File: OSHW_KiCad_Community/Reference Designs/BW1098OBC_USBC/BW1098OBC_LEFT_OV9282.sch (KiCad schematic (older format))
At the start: 20 parts, among them J2 BBR43-24KB533 for camera modu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

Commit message: Hierarchical pin/label/text fixes, ground/power nets fixed
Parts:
- C10, C11, C12, C7, C8, C9: symbol BW1098OBC_TopLevel-rescue:BW1098OBC_IMX378-rescue_GRM188R61A106ME69D--BW1098OBC_IMX378-SchDoc-rescue-BW1098OBC_IMX378-c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 -> depthAI_sch:GRM188R61A106ME69D
- FB4, FB5, FB6: symbol BW1098OBC_TopLevel-rescue:BW1098OBC_IMX378-rescue_2508056017Y2--BW1098OBC_IMX378-SchDoc-rescue-BW1098OBC_IMX378-cache -> depthAI_sch:2508056017Y2
- J2: symbol BW1098OBC_TopLevel-rescue:BW1098OBC_LEFT_OV9282-SchDoc-rescue_TG161B-201_Connector--BW1098OBC_LEFT_OV9282-cache -> depthAI_sch:TG161B-201_Connector
- R10, R4, R5, R6, R7, R8, R9: symbol BW1098OBC_TopLevel-rescue:BW1098OBC_LEFT_OV9282-SchDoc-rescue_CRCW06030000Z0EA--BW1098OBC_LEFT_OV9282-cache -> depthAI_sch:CRCW06030000Z0EA
- R11, R3: symbol BW1098OBC_TopLevel-rescue:BW1098OBC_IMX378-rescue_RC0402FR-1310KL--BW1098OBC_IMX378-SchDoc-rescue-BW1098OBC_IMX378-cache -> depthAI_sch:RC0402FR-1310KL
- R12: symbol BW1098OBC_TopLevel-rescue:BW1098OBC_LEFT_OV9282-SchDoc-rescue_CRCW04020000Z0ED--BW1098OBC_LEFT_OV9282-cache -> depthAI_sch:CRCW04020000Z0ED
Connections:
- net labels removed: FSIN1_IN, Parameter Set, Power_trace
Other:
- note added: "Parameter Set\nPower Trace"
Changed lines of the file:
@@
 Comment4 ""
 $EndDescr
-Text Label 9800 5800 0    60   ~ 0
+Text Label 10400 5800 0    60   ~ 0
 STROBE1
 Text Notes 6600 900  0    60   ~ 0
@@
 Text Label 13500 3600 0    60   ~ 0
 I2C2_SCL
-Text Label 9800 5200 0    60   ~ 0
+Text Label 10300 5200 0    60   ~ 0
 I2C2_SDA
-Text Label 9800 5100 0    60   ~ 0
+Text Label 10300 5100 0    60   ~ 0
 I2C2_SCL
 Text Notes 800  6550 0    60   ~ 0
@@
 	1    0    0    -1
 $EndComp
-Text Label 9800 5400 0    60   ~ 0
-FSIN1_IN
-Text Label 7150 7050 1    70   ~ 0
-Parameter Set
-Text Label 7250 7050 1    70   ~ 0
-Power_trace
-Text Label 8450 7050 1    70   ~ 0
-Parameter Set
-Text Label 8550 7050 1    70   ~ 0
-Power_trace
-Text Label 9750 7050 1    70   ~ 0
-Parameter Set
-Text Label 9850 7050 1    70   ~ 0
-Power_trace
 Text Label 9440 7440 0    70   ~ 0
 10V
@@
 	10300 5200 9300 5200
 Wire Wire Line
-	9300 4800 10300 4800
-Wire Wire Line
 	7500 5200 6200 5200
 Wire Wire Line
@@
 Wire Wire Line
 	800  6650 1500 6650
-Wire Wire Line
-	11400 5400 11000 5400
 Wire Wire Line
 	13300 3600 14100 3600
@@
 Connection ~ 9650 7450
 $Comp
-L BW1098OBC_TopLevel-rescue:BW1098OBC_IMX378-rescue_2508056017Y2--BW1098OBC_IMX378-SchDoc-rescue-BW1098OBC_IMX378-cache FB4
+L depthAI_sch:2508056017Y2 FB4
 U 1 1 5FD53040
 P 1400 1000
@@
 $EndComp
 $Comp
-L BW1098OBC_TopLevel-rescue:BW1098OBC_IMX378-rescue_GRM188R61A106ME69D--BW1098OBC_IMX378-SchDoc-rescue-BW1098OBC_IMX378-cache C8
+L depthAI_sch:GRM188R61A106ME69D C8
 U 1 1 5FD5303F
 P 7450 7350
@@
 $EndComp
 $Comp
-L BW1098OBC_TopLevel-rescue:BW1098OBC_IMX378-rescue_GRM188R61A106ME69D--BW1098OBC_IMX378-SchDoc-rescue-BW1098OBC_IMX378-cache C7
+L depthAI_sch:GRM188R61A106ME69D C7
 U 1 1 5FD5303E
 P 6850 7350
@@
 $EndComp
 $Comp
-L BW1098OBC_TopLevel-rescue:BW1098OBC_IMX378-rescue_GRM188R61A106ME69D--BW1098OBC_IMX378-SchDoc-rescue-BW1098OBC_IMX378-cache C9
+L depthAI_sch:GRM188R61A106ME69D C9
 U 1 1 5FD5303D
 P 8150 7350
@@
 $EndComp
 $Comp
-L BW1098OBC_TopLevel-rescue:BW1098OBC_LEFT_OV9282-SchDoc-rescue_TG161B-201_Connector--BW1098OBC_LEFT_OV9282-cache J2
+L depthAI_sch:TG161B-201_Connector J2
 U 1 1 5FD5303C
 P 7500 4800
@@
 $EndComp
 $Comp
-L BW1098OBC_TopLevel-rescue:BW1098OBC_LEFT_OV9282-SchDoc-rescue_CRCW06030000Z0EA--BW1098OBC_LEFT_OV9282-cache R4
+L depthAI_sch:CRCW06030000Z0EA R4
 U 1 1 5FD5303B
 P 2000 6150
@@
 $EndComp
 $Comp
-L BW1098OBC_TopLevel-rescue:BW1098OBC_LEFT_OV9282-SchDoc-rescue_CRCW06030000Z0EA--BW1098OBC_LEFT_OV9282-cache R7
+L depthAI_sch:CRCW06030000Z0EA R7
 U 1 1 5FD5303A
 P 2500 6150
@@
 $EndComp
 $Comp
-L BW1098OBC_TopLevel-rescue:BW1098OBC_LEFT_OV9282-SchDoc-rescue_CRCW06030000Z0EA--BW1098OBC_LEFT_OV9282-cache R10
+L depthAI_sch:CRCW06030000Z0EA R10
 U 1 1 5FD53039
 P 3000 6150
@@
 $EndComp
 $Comp
-L BW1098OBC_TopLevel-rescue:BW1098OBC_LEFT_OV9282-SchDoc-rescue_CRCW06030000Z0EA--BW1098OBC_LEFT_OV9282-cache R8
+L depthAI_sch:CRCW06030000Z0EA R8
 U 1 1 5FD53038
 P 2550 5700
@@
 $EndComp
 $Comp
-L BW1098OBC_TopLevel-rescue:BW1098OBC_LEFT_OV9282-SchDoc-rescue_CRCW06030000Z0EA--BW1098OBC_LEFT_OV9282-cache R5
+L depthAI_sch:CRCW06030000Z0EA R5
 U 1 1 5FD53037
 P 2050 5700
@@
 $EndComp
 $Comp
-L BW1098OBC_TopLevel-rescue:BW1098OBC_LEFT_OV9282-SchDoc-rescue_CRCW06030000Z0EA--BW1098OBC_LEFT_OV9282-cache R9
+L depthAI_sch:CRCW06030000Z0EA R9
 U 1 1 5FD53036
 P 2550 6200
@@
 $EndComp
 $Comp
-L BW1098OBC_TopLevel-rescue:BW1098OBC_IMX378-rescue_2508056017Y2--BW1098OBC_IMX378-SchDoc-rescue-BW1098OBC_IMX378-cache FB5
+L depthAI_sch:2508056017Y2 FB5
 U 1 1 5FD53035
 P 1400 1300
@@
 $EndComp
 $Comp
-L BW1098OBC_TopLevel-rescue:BW1098OBC_LEFT_OV9282-SchDoc-rescue_CRCW06030000Z0EA--BW1098OBC_LEFT_OV9282-cache R6
+L depthAI_sch:CRCW06030000Z0EA R6
 U 1 1 5FD53034
 P 2050 6200
@@
 $EndComp
 $Comp
-L BW1098OBC_TopLevel-rescue:BW1098OBC_IMX378-rescue_2508056017Y2--BW1098OBC_IMX378-SchDoc-rescue-BW1098OBC_IMX378-cache FB6
+L depthAI_sch:2508056017Y2 FB6
 U 1 1 5FD53033
 P 1400 1600
@@
 $EndComp
 $Comp
-L BW1098OBC_TopLevel-rescue:BW1098OBC_IMX378-rescue_RC0402FR-1310KL--BW1098OBC_IMX378-SchDoc-rescue-BW1098OBC_IMX378-cache R3
+L depthAI_sch:RC0402FR-1310KL R3
 U 1 1 5FD53032
 P 1500 6650
@@
 $EndComp
 $Comp
-L BW1098OBC_TopLevel-rescue:BW1098OBC_IMX378-rescue_RC0402FR-1310KL--BW1098OBC_IMX378-SchDoc-rescue-BW1098OBC_IMX378-cache R11
+L depthAI_sch:RC0402FR-1310KL R11
 U 1 1 5FD53031
 P 10600 5000
 F 0 "R11" H 10690 5030 60  0000 L BNN
-F 1 "10K 0402" H 10690 4870 60  0000 L BNN
+F 1 "10K 0402" H 10700 5100 60  0000 L BNN
 F 2 "" H 10690 4870 60  0001 C CNN
 F 3 "" H 10690 4870 60  0000 C CNN
@@
 $EndComp
 $Comp
-L BW1098OBC_TopLevel-rescue:BW1098OBC_LEFT_OV9282-SchDoc-rescue_CRCW04020000Z0ED--BW1098OBC_LEFT_OV9282-cache R12
+L depthAI_sch:CRCW04020000Z0ED R12
 U 1 1 5FD53030
 P 10600 5400
@@
 $EndComp
 $Comp
-L BW1098OBC_TopLevel-rescue:BW1098OBC_IMX378-rescue_GRM188R61A106ME69D--BW1098OBC_IMX378-SchDoc-rescue-BW1098OBC_IMX378-cache C11
+L depthAI_sch:GRM188R61A106ME69D C11
 U 1 1 5FD5302F
 P 9350 7350
@@
 $EndComp
 $Comp
-L BW1098OBC_TopLevel-rescue:BW1098OBC_IMX378-rescue_GRM188R61A106ME69D--BW1098OBC_IMX378-SchDoc-rescue-BW1098OBC_IMX378-cache C12
+L depthAI_sch:GRM188R61A106ME69D C12
 U 1 1 5FD5302E
 P 9950 7350
@@
 $EndComp
 $Comp
-L BW1098OBC_TopLevel-rescue:BW1098OBC_IMX378-rescue_GRM188R61A106ME69D--BW1098OBC_IMX378-SchDoc-rescue-BW1098OBC_IMX378-cache C10
+L depthAI_sch:GRM188R61A106ME69D C10
 U 1 1 5FD5302D
 P 8750 7350
@@
 Text HLabel 9700 5600 2    79   BiDi ~ 0
 2V8_L
-Text HLabel 11350 5400 2    79   BiDi ~ 0
-FSIN1
 Text GLabel 3000 5150 2    60   Output ~ 0
 FSIN2
@@
 Text GLabel 13750 5150 2    79   UnSpc ~ 0
 CAM_B_CLK_OUT
+Wire Wire Line
+	11400 5400 11000 5400
+Text Label 11400 5400 0    60   ~ 0
+FSIN1
+Wire Wire Line
+	9800 4800 9300 4800
+Text Notes 9800 7050 1    60   ~ 0
+Parameter Set\nPower Trace
+Text Notes 7300 7050 1    60   ~ 0
+Parameter Set\nPower Trace
+Text Notes 8600 7050 1    60   ~ 0
+Parameter Set\nPower Trace
 $EndSCHEMATC

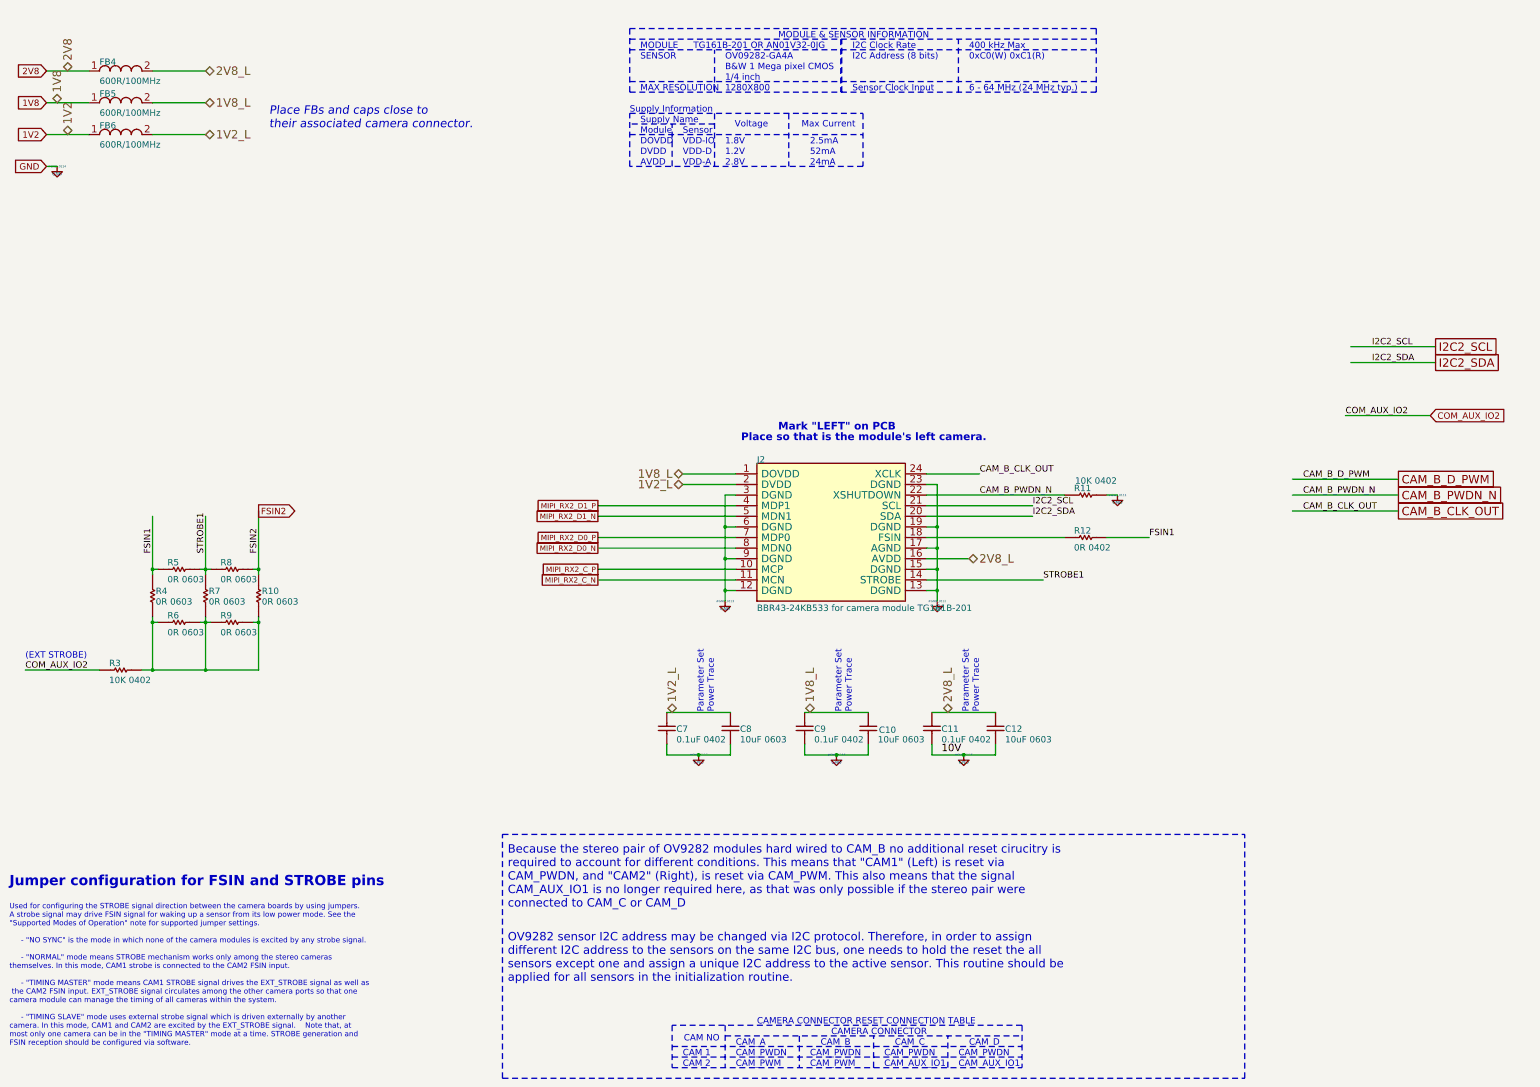
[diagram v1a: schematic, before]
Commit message: schematic ready for review
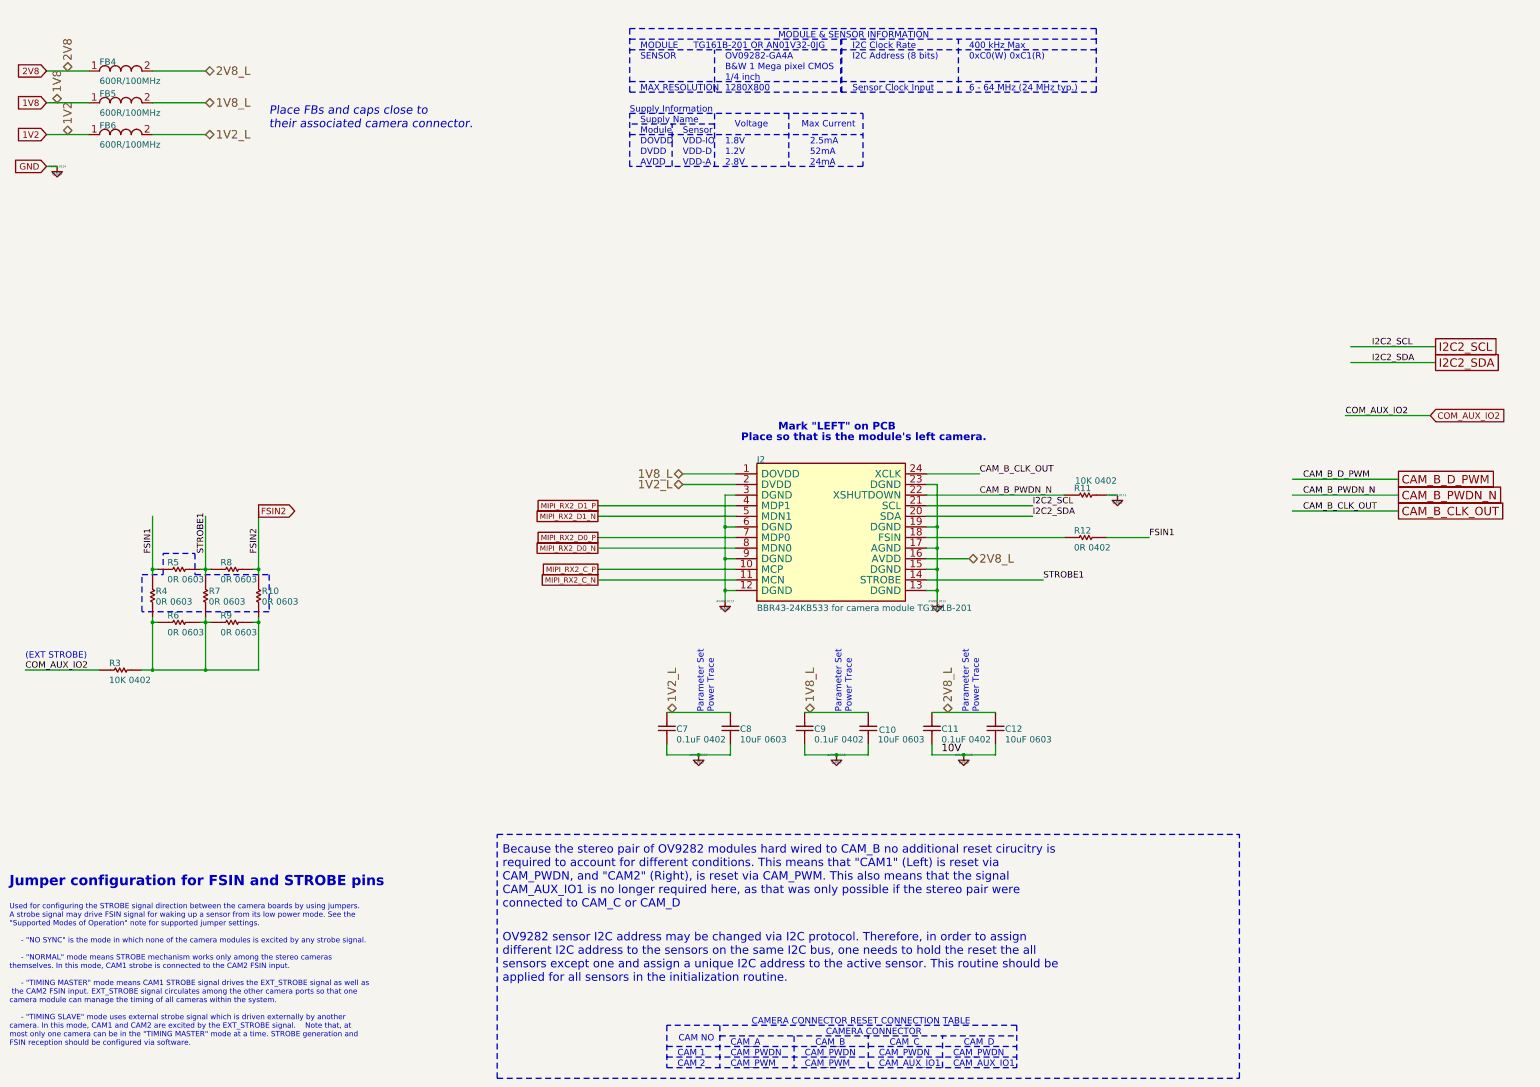
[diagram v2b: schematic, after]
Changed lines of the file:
@@
 Jumper configuration for FSIN and STROBE pins
 Wire Notes Line
-	5300 10500 5300 8200
+	5250 10500 5250 8200
 Wire Notes Line
-	5300 10500 12300 10500
+	5250 10500 12250 10500
 Wire Notes Line
-	5300 8200 12300 8200
+	5250 8200 12250 8200
 Wire Notes Line
-	12300 10500 12300 8200
+	12250 10500 12250 8200
 Text Notes 7900 4400 0    72   ~ 14
 Mark "LEFT" on PCB
-Text Notes 7010 10160 0    60   ~ 0
+Text Notes 6960 10160 0    60   ~ 0
 CAM NO
-Text Notes 7000 10300 0    60   ~ 0
+Text Notes 6950 10300 0    60   ~ 0
 CAM 1
-Text Notes 7000 10400 0    60   ~ 0
+Text Notes 6950 10400 0    60   ~ 0
 CAM 2
 Wire Notes Line
-	10200 10000 6900 10000
-Text Notes 7500 10200 0    60   ~ 0
+	10150 10000 6850 10000
+Text Notes 7450 10200 0    60   ~ 0
 CAM_A
 Wire Notes Line
-	8800 10400 8800 10100
+	8750 10400 8750 10100
 Wire Notes Line
-	9500 10400 9500 10100
-Text Notes 8400 10100 0    60   ~ 0
+	9450 10400 9450 10100
+Text Notes 8350 10100 0    60   ~ 0
 CAMERA CONNECTOR
-Text Notes 7500 10300 0    60   ~ 0
+Text Notes 7450 10300 0    60   ~ 0
 CAM_PWDN
-Text Notes 8200 10300 0    60   ~ 0
+Text Notes 8150 10300 0    60   ~ 0
 CAM_PWDN
-Text Notes 7500 10400 0    60   ~ 0
+Text Notes 7450 10400 0    60   ~ 0
 CAM_PWM
-Text Notes 8200 10400 0    60   ~ 0
+Text Notes 8150 10400 0    60   ~ 0
 CAM_PWM
-Text Notes 8900 10300 0    60   ~ 0
+Text Notes 8850 10300 0    60   ~ 0
 CAM_PWDN
-Text Notes 8900 10400 0    60   ~ 0
+Text Notes 8850 10400 0    60   ~ 0
 CAM_AUX_IO1
-Text Notes 9600 10400 0    60   ~ 0
+Text Notes 9550 10400 0    60   ~ 0
 CAM_AUX_IO1
-Text Notes 9600 10300 0    60   ~ 0
+Text Notes 9550 10300 0    60   ~ 0
 CAM_PWDN
-Text Notes 8300 10200 0    60   ~ 0
+Text Notes 8250 10200 0    60   ~ 0
 CAM_B
-Text Notes 9000 10200 0    60   ~ 0
+Text Notes 8950 10200 0    60   ~ 0
 CAM_C
-Text Notes 9700 10200 0    60   ~ 0
+Text Notes 9650 10200 0    60   ~ 0
 CAM_D
-Text Notes 7700 10000 0    60   ~ 0
+Text Notes 7650 10000 0    60   ~ 0
 CAMERA CONNECTOR RESET CONNECTION TABLE
 $Comp
@@
 	6500 1600 8700 1600
 Wire Notes Line
-	6900 10200 10200 10200
+	6850 10200 10150 10200
 Wire Notes Line
-	8100 10100 8100 10400
+	8050 10100 8050 10400
 Wire Notes Line
-	6900 10000 6900 10400
+	6850 10000 6850 10400
 Wire Notes Line
-	6900 10400 10200 10400
+	6850 10400 10150 10400
 Wire Notes Line
-	6900 10300 10200 10300
+	6850 10300 10150 10300
 Wire Notes Line
-	10200 10000 10200 10400
+	10150 10000 10150 10400
 Wire Notes Line
-	7400 10000 7400 10400
+	7350 10000 7350 10400
 Wire Notes Line
-	7400 10100 10200 10100
+	7350 10100 10150 10100
 Text GLabel 6200 5100 0    50   UnSpc ~ 0
 MIPI_RX2_D1_P
@@
 Text Notes 650  10200 0    50   ~ 0
 Used for configuring the STROBE signal direction between the camera boards by using jumpers. \nA strobe signal may drive FSIN signal for waking up a sensor from its low power mode. See the \n"Supported Modes of Operation" note for supported jumper settings.     \n \n     - "NO SYNC" is the mode in which none of the camera modules is excited by any strobe signal.  \n   \n     - "NORMAL" mode means STROBE mechanism works only among the stereo cameras \nthemselves. In this mode, CAM1 strobe is connected to the CAM2 FSIN input.      \n\n     - "TIMING MASTER" mode means CAM1 STROBE signal drives the EXT_STROBE signal as well as\n the CAM2 FSIN input. EXT_STROBE signal circulates among the other camera ports so that one \ncamera module can manage the timing of all cameras within the system.    \n\n     - "TIMING SLAVE" mode uses external strobe signal which is driven externally by another \ncamera. In this mode, CAM1 and CAM2 are excited by the EXT_STROBE signal.    Note that, at \nmost only one camera can be in the "TIMING MASTER" mode at a time. STROBE generation and \nFSIN reception should be configured via software.  \n
-Text Notes 5350 9600 0    79   ~ 0
+Text Notes 5300 9600 0    79   ~ 0
 OV9282 sensor I2C address may be changed via I2C protocol. Therefore, in order to assign \ndifferent I2C address to the sensors on the same I2C bus, one needs to hold the reset the all \nsensors except one and assign a unique I2C address to the active sensor. This routine should be \napplied for all sensors in the initialization routine.
-Text Notes 5350 8900 0    79   ~ 0
+Text Notes 5300 8900 0    79   ~ 0
 Because the stereo pair of OV9282 modules hard wired to CAM_B no additional reset cirucitry is \nrequired to account for different conditions. This means that "CAM1" (Left) is reset via \nCAM_PWDN, and "CAM2" (Right), is reset via CAM_PWM. This also means that the signal \nCAM_AUX_IO1 is no longer required here, as that was only possible if the stereo pair were \nconnected to CAM_C or CAM_D
 $Bitmap
@@
 Text Notes 8600 7050 1    60   ~ 0
 Parameter Set\nPower Trace
+Wire Notes Line width 16 style dash_dot rgb(255, 0, 0)
+	3100 5750 3100 6100
+Wire Notes Line width 16 style dash_dot rgb(255, 0, 0)
+	3100 6100 1900 6100
+Wire Notes Line width 16 style dash_dot rgb(255, 0, 0)
+	1900 6100 1900 5750
+Wire Notes Line width 16 style dash_dot rgb(255, 0, 0)
+	1900 5750 2100 5750
+Wire Notes Line width 16 style dash_dot rgb(255, 0, 0)
+	2100 5750 2100 5550
+Wire Notes Line width 16 style dash_dot rgb(255, 0, 0)
+	2100 5550 2400 5550
+Wire Notes Line width 16 style dash_dot rgb(255, 0, 0)
+	2400 5550 2400 5750
+Wire Notes Line width 16 style dash_dot rgb(255, 0, 0)
+	2400 5750 3100 5750
 $EndSCHEMATC
